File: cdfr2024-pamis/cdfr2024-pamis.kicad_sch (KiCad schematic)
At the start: 15 parts, among them J1 Connecteur batterie, J2 Connecteur Bouton, J4 Moteur Droit, J5 Connecteur ToF, J7 Moteur Gauche, J8 Connecteur RF, U1 ESP32-DEVKIT-V1, U1 LM317_SOT-223, U4 Driver Moteur Droit, U5 Driver Moteur Gauche

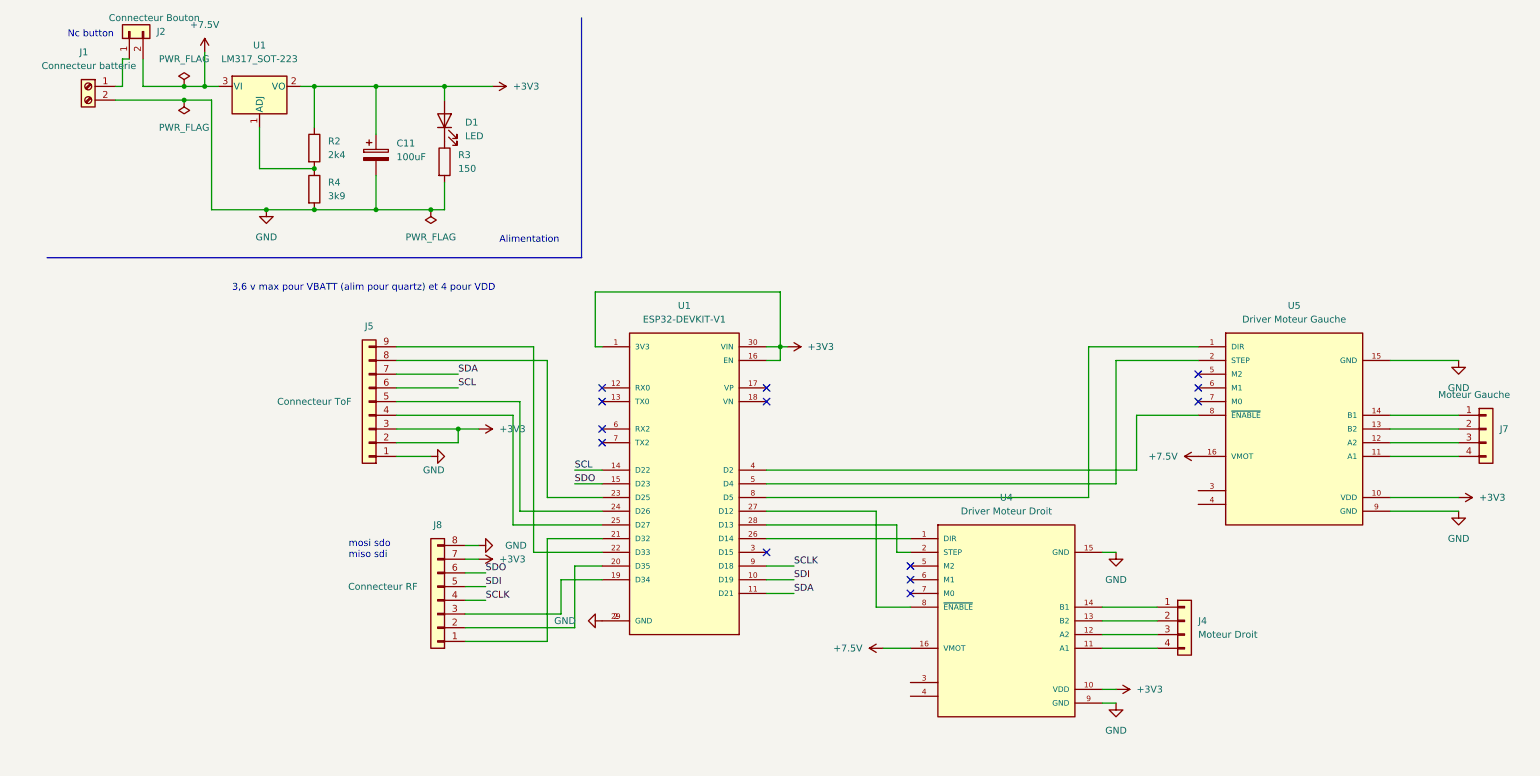
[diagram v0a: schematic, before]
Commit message: carte pamis
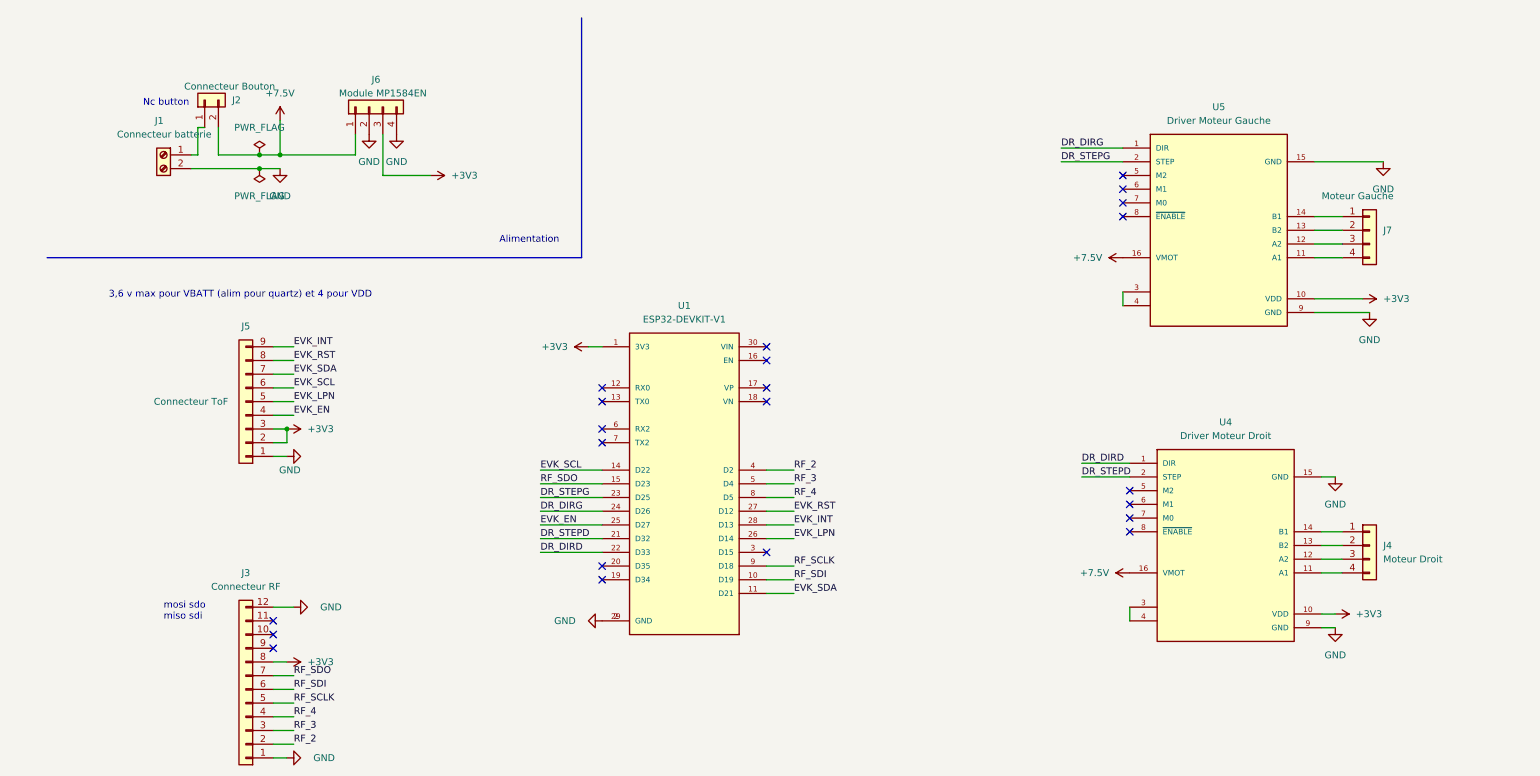
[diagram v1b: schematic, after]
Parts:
- removed C11: 100uF, Capacitor_SMD:CP_Elec_10x10.5, symbol Device:C_Polarized
- removed D1: LED, LED_SMD:LED_0805_2012Metric_Pad1.15x1.40mm_HandSolder, symbol Device:LED
- removed J8: Connecteur RF, Connector_PinHeader_2.54mm:PinHeader_1x08_P2.54mm_Vertical, symbol Connector_Generic:Conn_01x08
- removed R2: 2k4, Resistor_SMD:R_0805_2012Metric_Pad1.20x1.40mm_HandSolder, symbol Device:R
- removed R3: 150, Resistor_SMD:R_0805_2012Metric_Pad1.20x1.40mm_HandSolder, symbol Device:R
- removed R4: 3k9, Resistor_SMD:R_0805_2012Metric_Pad1.20x1.40mm_HandSolder, symbol Device:R
- removed U1: LM317_SOT-223, Package_TO_SOT_SMD:SOT-223-3_TabPin2, symbol Regulator_Linear:LM317_SOT-223
- added J3: Connecteur RF, Connector_PinHeader_2.54mm:PinHeader_1x12_P2.54mm_Vertical, symbol Connector_Generic:Conn_01x12
- added J6: Module MP1584EN, MP1584EN_Module:SRT_MPT1584EN_Module, symbol Connector_Generic:Conn_01x04
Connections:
- net +3V3: now also J3.8 (Pin_8), J6.3 (Pin_3); no longer U1.16 (EN), U1.30 (VIN)
- net +7.5V: now also J6.1 (Pin_1)
- net GND: now also J3.1 (Pin_1), J3.12 (Pin_12), J6.2 (Pin_2), J6.4 (Pin_4)
- net DR_DIRD: now reaches U4.1 (DIR)
- net DR_DIRD: now also U1.22 (D33); no longer U1.26 (D14)
- net DR_STEPD: now reaches U4.2 (STEP)
- net DR_STEPD: now also U1.21 (D32); no longer U1.28 (D13)
- net at U4.3: now also U4.4
- net at U4.8 (~{ENABLE}): no longer U1.27 (D12)
- net EVK_INT: now reaches J5.9 (Pin_9)
- net EVK_INT: now also U1.28 (D13); no longer U1.22 (D33)
- net DR_STEPG: now reaches U1.23 (D25)
- net DR_STEPG: now also U5.2 (STEP); no longer J5.8 (Pin_8)
- net DR_DIRG: now reaches U1.24 (D26)
- net DR_DIRG: now also U5.1 (DIR); no longer J5.5 (Pin_5)
- net EVK_EN: now reaches J5.4 (Pin_4), U1.25 (D27)
- net at U5.8 (~{ENABLE}): no longer U1.4 (D2)
- net RF_3: now reaches U1.5 (D4)
- net RF_3: now also J3.3 (Pin_3); no longer U5.2 (STEP)
- net RF_4: now reaches U1.8 (D5)
- net RF_4: now also J3.4 (Pin_4); no longer U5.1 (DIR)
- net at U5.3: now also U5.4
- net SCL renamed EVK_SCL
- net SCLK renamed RF_SCLK
- net RF_SCLK: now also J3.5 (Pin_5)
- net SDA renamed EVK_SDA
- net SDI renamed RF_SDI
- net RF_SDI: now also J3.6 (Pin_6)
- net SDO renamed RF_SDO
- net RF_SDO: now also J3.7 (Pin_7)
- new net EVK_LPN: J5.5 (Pin_5), U1.26 (D14)
- new net EVK_RST: J5.8 (Pin_8), U1.27 (D12)
- new net RF_2: J3.2 (Pin_2), U1.4 (D2)
- no-connect marks 13 -> 22
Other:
- moved on the sheet: J1, J2, J4, J5, J7, U4, U5
